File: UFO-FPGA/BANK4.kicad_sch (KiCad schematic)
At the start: 20 parts, among them SW1 SW_Push_DPDT, SW2 SW_DIP_x01, U1 ICE40HX8K-BG121

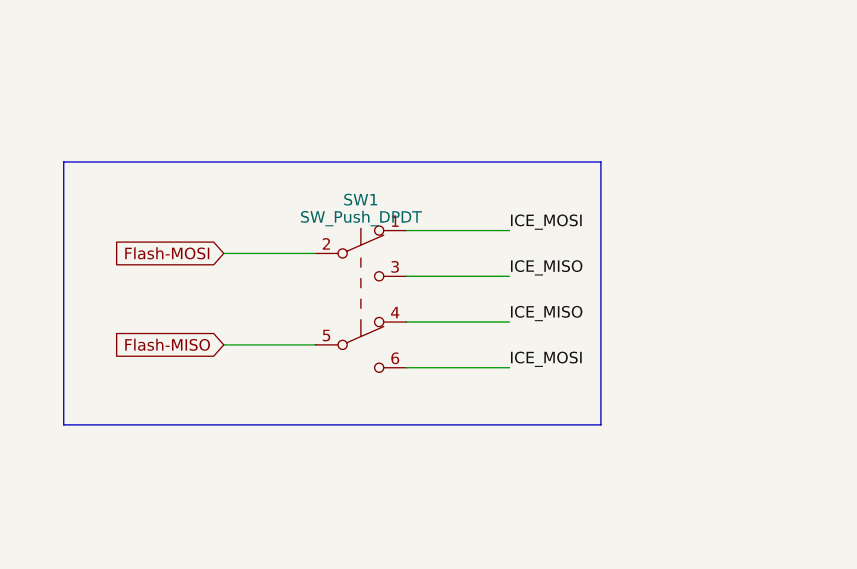
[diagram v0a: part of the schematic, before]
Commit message: Explainer
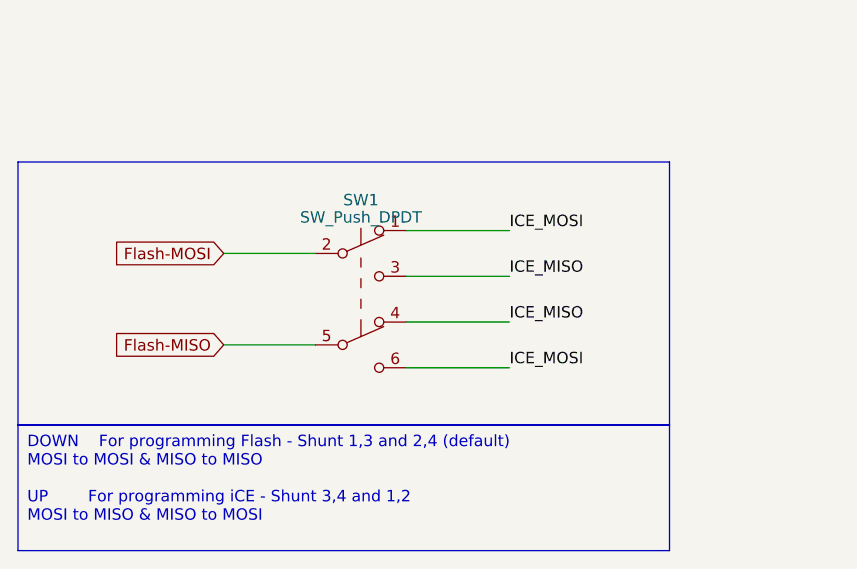
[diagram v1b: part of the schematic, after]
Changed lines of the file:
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@@
     (stroke (width 0) (type default))
   )
-  (rectangle (start 39.37 148.59) (end 99.06 177.8)
+  (rectangle (start 34.29 148.59) (end 106.68 177.8)
     (stroke (width 0) (type default))
     (fill (type none))
   )
+  (text_box "DOWN	For programming Flash - Shunt 1,3 and 2,4 (default)\nMOSI to MOSI & MISO to MISO\n\nUP		For programming iCE - Shunt 3,4 and 1,2\nMOSI to MISO & MISO to MOSI"
+    (at 34.29 177.8 0) (size 72.39 13.97)
+    (stroke (width 0) (type default))
+    (fill (type none))
+    (effects (font (size 1.27 1.27)) (justify left top))
+  )
   (label "ICE_MISO" (at 88.9 166.37 0) (fields_autoplaced)
